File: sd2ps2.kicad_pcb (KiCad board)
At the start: 2 copper layers, 36 x 52.5 mm, 12 parts, among them J1 , J2 DM3AT-SF-PEJM5, Q1 DTC114T, Q2 DTC114T

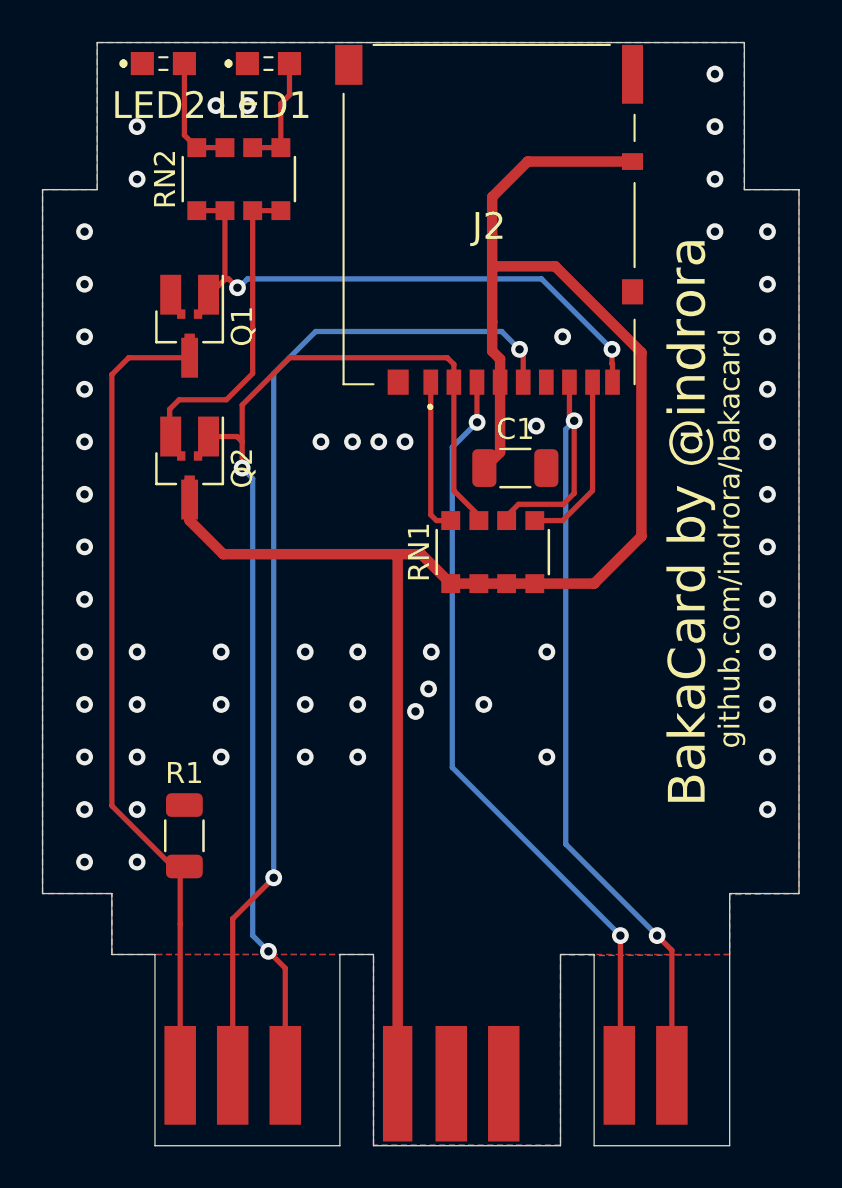
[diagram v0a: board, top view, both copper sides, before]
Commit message: rev c
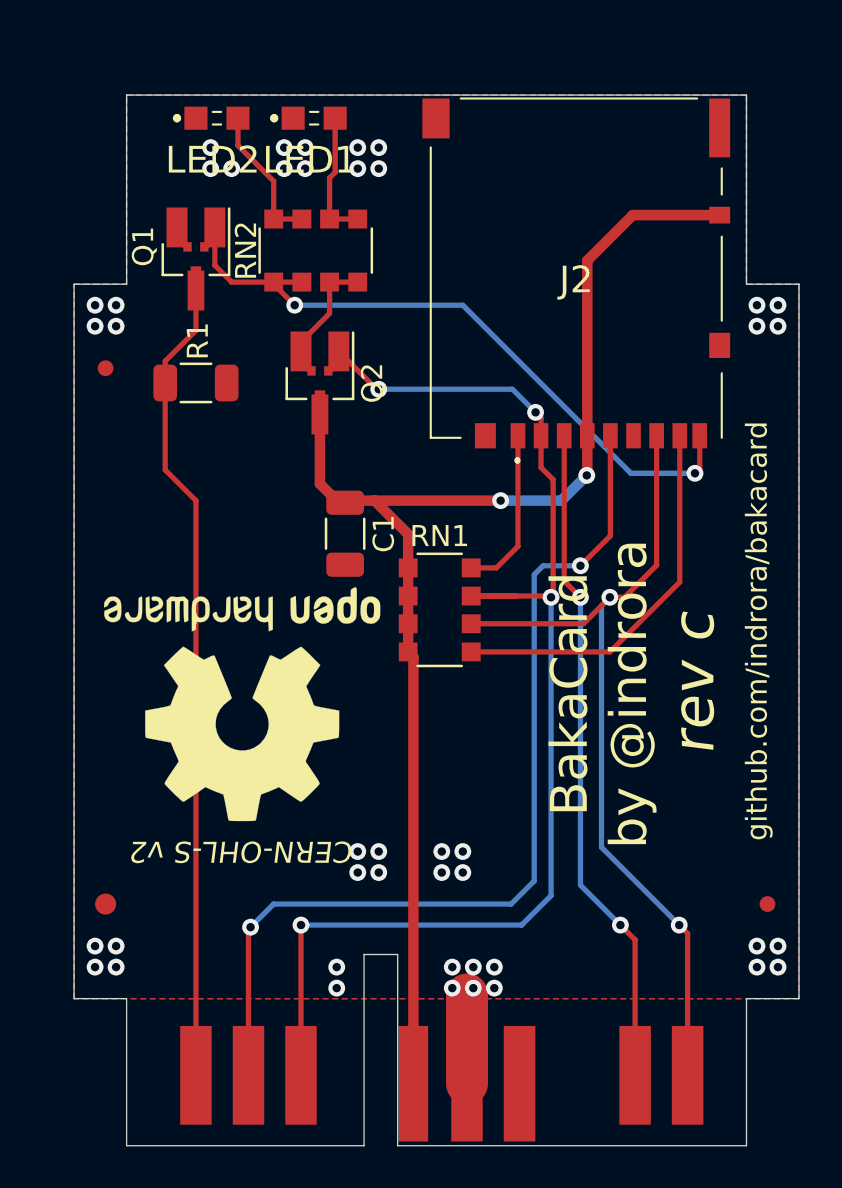
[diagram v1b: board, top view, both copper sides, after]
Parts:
- added FID1: Fiducial, Fiducial:Fiducial_0.75mm_Mask1.5mm, F.Cu at (200.0, 117.0)
- added FID2: Fiducial, Fiducial:Fiducial_0.75mm_Mask1.5mm, F.Cu at (168.5, 91.5)
- added FID3: Fiducial, Fiducial:Fiducial_1mm_Mask2mm, F.Cu at (168.5, 117.0)
- REF**: value OSHW-Logo2_7.3x6mm_SilkScreen -> OSHW-Logo2_14.6x12mm_SilkScreen; footprint Symbol:OSHW-Logo2_7.3x6mm_SilkScreen -> Symbol:OSHW-Logo2_14.6x12mm_SilkScreen; moved to F.Cu
- moved R1 21.6 mm to (172.8, 92.2), turned to 0 degrees
- moved REF** 20.2 mm to (175.0, 107.5), turned to 180 degrees
- moved C1 8.68 mm to (179.9, 99.4), turned to -90 degrees
- moved Q2 7.41 mm to (178.7, 92.2)
- moved RN2 5.00 mm to (178.5, 85.9)
- moved J2 4.87 mm to (190.9, 87.3)
- moved RN1 3.73 mm to (184.4, 103.0), turned to 0 degrees
- moved LED2 3.64 mm to (173.8, 79.6)
- moved G*** 3.45 mm to (184.2, 103.0)
- moved LED1 3.39 mm to (178.4, 79.6)
- moved Q1 3.21 mm to (172.8, 86.3)
- moved J1 0.75 mm to (184.2, 128.5)
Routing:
- net +3V3: track 88.2 -> 62.8 mm, vias 0 -> 2
- net Net-(Q2-Pad2): track 15.0 -> 4.75 mm
- net Net-(J2-Pad8): track 8.50 -> 18.3 mm
- net /CS: track 53.6 -> 59.6 mm, vias 2 -> 4
- net /DI: track 36.8 -> 31.8 mm
- net /CD: track 27.4 -> 32.0 mm
- net GND: track 0.00 -> 4.25 mm, vias 59 -> 43
- net /CLK: track 48.7 -> 45.2 mm
- net /DO: track 42.7 -> 40.8 mm
- net Net-(LED2-Pad2): track 5.58 -> 6.84 mm
- net Net-(LED1-Pad2): track 5.51 -> 6.25 mm
- net /ACK: track 39.2 -> 38.6 mm
- net Net-(J2-Pad1): track 7.38 -> 7.91 mm
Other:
- board size 36 x 52.5 mm -> 34.5 x 50 mm
- board text added: "dedicated to Near"
- board text added: "rev c"
- board text removed: "rev b"
